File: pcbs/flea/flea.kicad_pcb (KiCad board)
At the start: 2 copper layers, 116.6 x 85.2 mm, 19 parts, among them SW1 SW_PUSH, SW10 SW_PUSH, SW11 SW_PUSH, SW12 SW_PUSH, SW13 SW_PUSH, SW14 SW_PUSH, SW15 SW_PUSH, SW2 SW_PUSH, SW3 SW_PUSH, SW4 SW_PUSH, SW5 SW_PUSH, SW6 SW_PUSH, SW7 SW_PUSH, SW8 SW_PUSH, SW9 SW_PUSH, U1 ProMicro

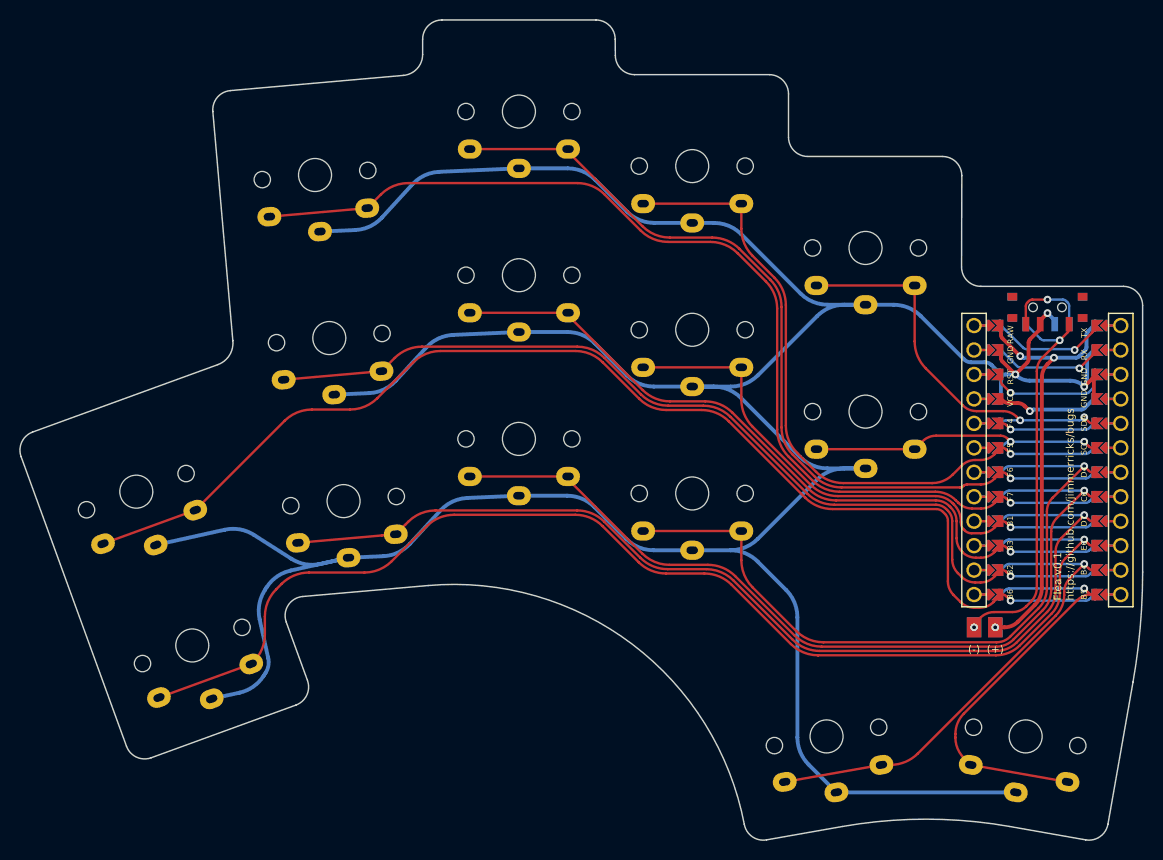
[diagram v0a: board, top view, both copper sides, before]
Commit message: Update flea edge
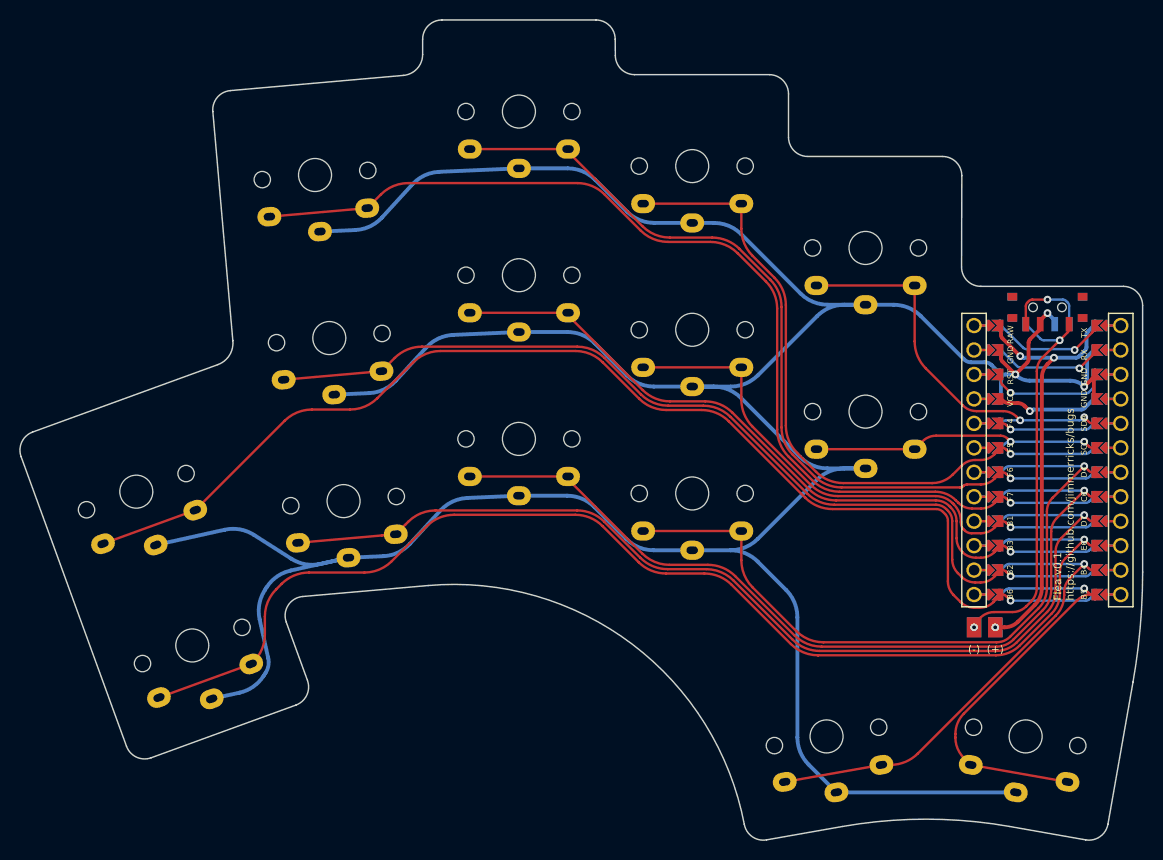
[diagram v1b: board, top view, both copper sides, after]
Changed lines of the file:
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@@
-(kicad_pcb (version 20210925) (generator pcbnew)
+(kicad_pcb (version 20211014) (generator pcbnew)
   (general
     (thickness 1.6)
@@
   )
   (gr_line (start 147.747178 76.077192) (end 147.749256 103.754181) (layer "Edge.Cuts") (width 0.15))
-  (gr_arc (start 90.967358 48.411064) (end 92.967358 48.411063) (angle -90) (layer "Edge.Cuts") (width 0.15))
+  (gr_arc (start 90.967357 46.411064) (mid 92.381571 46.99685) (end 92.967358 48.411063) (layer "Edge.Cuts") (width 0.15))
   (gr_line (start 32.460178 89.20989) (end 51.698026 82.207748) (layer "Edge.Cuts") (width 0.15))
-  (gr_arc (start 74.967354 48.411069) (end 74.967353 46.411069) (angle -90) (layer "Edge.Cuts") (width 0.15))
+  (gr_arc (start 72.967354 48.41107) (mid 73.55314 46.996856) (end 74.967353 46.411069) (layer "Edge.Cuts") (width 0.15))
   (gr_line (start 31.264832 91.773313) (end 42.209651 121.843944) (layer "Edge.Cuts") (width 0.15))
-  (gr_arc (start 130.941303 72.077188) (end 128.941306 72.07719) (angle -90) (layer "Edge.Cuts") (width 0.15))
+  (gr_arc (start 130.941305 74.077185) (mid 129.527093 73.491401) (end 128.941306 72.07719) (layer "Edge.Cuts") (width 0.15))
   (gr_line (start 110.966787 54.088034) (end 110.967178 58.587188) (layer "Edge.Cuts") (width 0.15))
   (gr_line (start 133.947659 130.176564) (end 141.826123 131.565744) (layer "Edge.Cuts") (width 0.15))
   (gr_line (start 108.689942 131.565986) (end 116.568399 130.176802) (layer "Edge.Cuts") (width 0.15))
-  (gr_arc (start 53.167635 55.737651) (end 52.993326 53.745266) (angle -90) (layer "Edge.Cuts") (width 0.15))
-  (gr_arc (start 70.784999 49.993054) (end 70.975227 52.16736) (angle -84.99985992) (layer "Edge.Cuts") (width 0.15))
-  (gr_arc (start 108.342642 129.596367) (end 106.373027 129.943665) (angle -90) (layer "Edge.Cuts") (width 0.15))
-  (gr_arc (start 60.673589 108.274936) (end 60.518025 106.290257) (angle -105.5192513) (layer "Edge.Cuts") (width 0.15))
+  (gr_arc (start 51.17525 55.91196) (mid 51.635551 54.452077) (end 52.993326 53.745266) (layer "Edge.Cuts") (width 0.15))
+  (gr_arc (start 72.967611 49.993058) (mid 72.394188 51.467606) (end 70.975227 52.16736) (layer "Edge.Cuts") (width 0.15))
+  (gr_arc (start 108.68994 131.565982) (mid 107.195491 131.234672) (end 106.373027 129.943665) (layer "Edge.Cuts") (width 0.15))
+  (gr_arc (start 58.802893 108.955853) (mid 58.999438 107.197732) (end 60.518025 106.290257) (layer "Edge.Cuts") (width 0.15))
   (gr_line (start 60.518025 106.290257) (end 73.552042 105.149929) (layer "Edge.Cuts") (width 0.15))
-  (gr_arc (start 33.144216 91.089274) (end 32.460178 89.20989) (angle -90) (layer "Edge.Cuts") (width 0.15))
-  (gr_line (start 112.967179 60.587188) (end 126.966962 60.58741) (layer "Edge.Cuts") (width 0.15))
-  (gr_arc (start 142.173419 129.596128) (end 141.826123 131.565744) (angle -90) (layer "Edge.Cuts") (width 0.15))
+  (gr_arc (start 31.264832 91.773312) (mid 31.331603 90.244037) (end 32.460178 89.20989) (layer "Edge.Cuts") (width 0.15))
+  (gr_line (start 112.967179 60.587188) (end 126.966959 60.587398) (layer "Edge.Cuts") (width 0.15))
+  (gr_arc (start 144.143035 129.943424) (mid 143.320572 131.234432) (end 141.826123 131.565744) (layer "Edge.Cuts") (width 0.15))
   (gr_line (start 144.143032 129.943424) (end 146.748563 115.17185) (layer "Edge.Cuts") (width 0.15))
-  (gr_arc (start 125.258705 179.453893) (end 133.947659 130.176564) (angle -20.00164516) (layer "Edge.Cuts") (width 0.15))
-  (gr_line (start 130.941304 74.077179) (end 145.747175 74.077192) (layer "Edge.Cuts") (width 0.15))
-  (gr_arc (start 126.966958 62.587404) (end 128.966964 62.587405) (angle -90) (layer "Edge.Cuts") (width 0.15))
-  (gr_arc (start 44.089034 121.159907) (end 42.209651 121.843944) (angle -90) (layer "Edge.Cuts") (width 0.15))
-  (gr_arc (start 112.967177 58.587189) (end 110.967178 58.587188) (angle -90) (layer "Edge.Cuts") (width 0.15))
+  (gr_arc (start 116.568397 130.176803) (mid 125.258018 129.416377) (end 133.947659 130.176564) (layer "Edge.Cuts") (width 0.15))
+  (gr_line (start 130.941305 74.077185) (end 145.747176 74.077184) (layer "Edge.Cuts") (width 0.15))
+  (gr_arc (start 126.966959 60.587398) (mid 128.381177 61.173187) (end 128.966964 62.587405) (layer "Edge.Cuts") (width 0.15))
+  (gr_arc (start 44.773071 123.03929) (mid 43.243797 122.972519) (end 42.209651 121.843944) (layer "Edge.Cuts") (width 0.15))
+  (gr_arc (start 112.967176 60.587188) (mid 111.552963 60.001401) (end 110.967178 58.587188) (layer "Edge.Cuts") (width 0.15))
   (gr_line (start 94.981842 52.08814) (end 108.966789 52.088035) (layer "Edge.Cuts") (width 0.15))
-  (gr_arc (start 145.747173 76.077189) (end 147.747178 76.077192) (angle -90) (layer "Edge.Cuts") (width 0.15))
-  (gr_arc (start 94.981842 50.088139) (end 92.981845 50.08814) (angle -90) (layer "Edge.Cuts") (width 0.15))
+  (gr_arc (start 145.747176 74.077184) (mid 147.161392 74.662974) (end 147.747178 76.077192) (layer "Edge.Cuts") (width 0.15))
+  (gr_arc (start 94.981843 52.088136) (mid 93.567631 51.502351) (end 92.981845 50.08814) (layer "Edge.Cuts") (width 0.15))
   (gr_line (start 53.253324 79.711739) (end 51.175248 55.911961) (layer "Edge.Cuts") (width 0.15))
-  (gr_arc (start 50.882457 79.966988) (end 51.698026 82.207748) (angle -76.14476749) (layer "Edge.Cuts") (width 0.15))
-  (gr_arc (start 59.124579 115.687279) (end 59.808617 117.566666) (angle -90) (layer "Edge.Cuts") (width 0.15))
-  (gr_line (start 72.96735 48.411067) (end 72.967612 49.993053) (layer "Edge.Cuts") (width 0.15))
+  (gr_arc (start 53.253323 79.711743) (mid 52.906278 81.228061) (end 51.698026 82.207748) (layer "Edge.Cuts") (width 0.15))
+  (gr_arc (start 61.003966 115.003241) (mid 60.937194 116.532518) (end 59.808617 117.566666) (layer "Edge.Cuts") (width 0.15))
+  (gr_line (start 72.967354 48.41107) (end 72.967611 49.993058) (layer "Edge.Cuts") (width 0.15))
   (gr_line (start 74.967353 46.411069) (end 90.967361 46.411066) (layer "Edge.Cuts") (width 0.15))
   (gr_line (start 58.802893 108.955851) (end 61.003968 115.003239) (layer "Edge.Cuts") (width 0.15))
   (gr_line (start 52.993326 53.745266) (end 70.975227 52.16736) (layer "Edge.Cuts") (width 0.15))
-  (gr_arc (start 81.880446 103.733849) (end 146.748563 115.17185) (angle -9.982315587) (layer "Edge.Cuts") (width 0.15))
-  (gr_arc (start 76.227246 135.729039) (end 106.373027 129.943665) (angle -84.13604418) (layer "Edge.Cuts") (width 0.15))
-  (gr_arc (start 108.966787 54.088035) (end 110.966787 54.088034) (angle -90) (layer "Edge.Cuts") (width 0.15))
+  (gr_arc (start 147.749255 103.754181) (mid 147.497721 109.484822) (end 146.748563 115.17185) (layer "Edge.Cuts") (width 0.15))
+  (gr_arc (start 73.552042 105.149929) (mid 94.729692 111.23622) (end 106.373027 129.943665) (layer "Edge.Cuts") (width 0.15))
+  (gr_arc (start 108.966786 52.088035) (mid 110.381 52.673821) (end 110.966787 54.088034) (layer "Edge.Cuts") (width 0.15))
   (gr_line (start 128.966964 62.587405) (end 128.941306 72.07719) (layer "Edge.Cuts") (width 0.15))
   (gr_line (start 44.773073 123.039293) (end 59.808617 117.566666) (layer "Edge.Cuts") (width 0.15))
